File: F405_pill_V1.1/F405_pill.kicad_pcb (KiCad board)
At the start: 4 copper layers, 53.8 x 19.4 mm, 50 parts, among them J1 Conn_01x04_Male, J2 Conn_01x04_Male, J4 TYPE-C-31-M-12, U1 STM32F405RGTx, U2 MAX3051EKA+T, U3 LM1117-3.3, U4 STM32F405_pill, U5 HT7550-1, Y1 Crystal_GND24

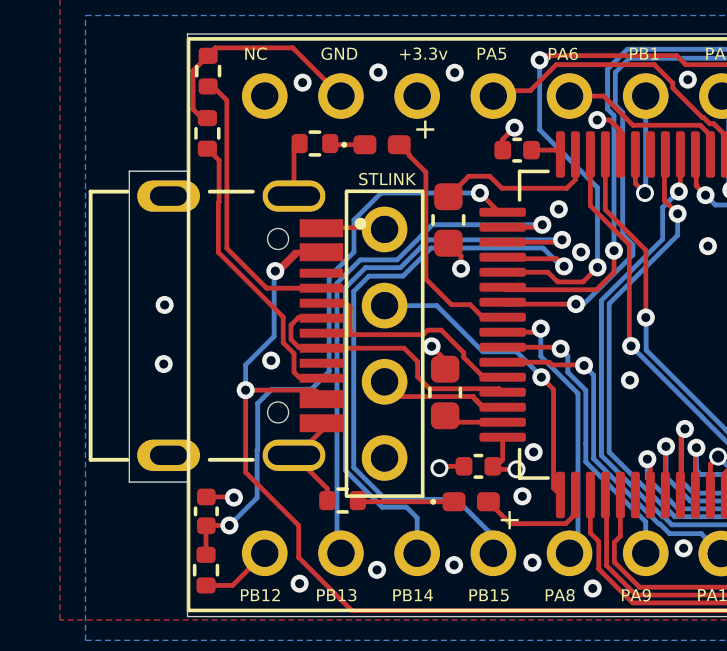
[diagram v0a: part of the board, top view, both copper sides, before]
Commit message: finalizing
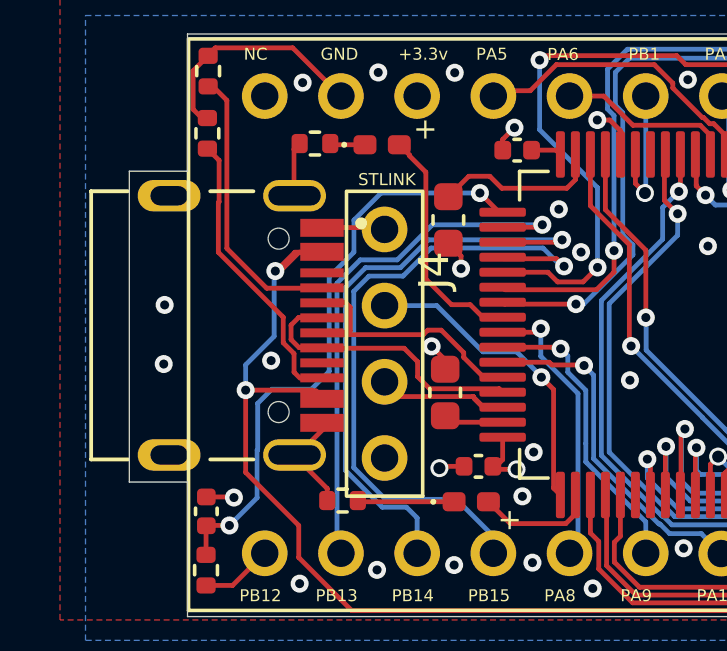
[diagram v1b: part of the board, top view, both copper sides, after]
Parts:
- D3: value RED_LED -> RED
- moved J4 2.52 mm to (98.2, 84.7)
